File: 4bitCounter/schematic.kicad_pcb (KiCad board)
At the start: 2 copper layers, 20 parts, among them J2 Conn_01x02_Pin, Q1 PN2222A, U1 NE555P, U3 74LS161

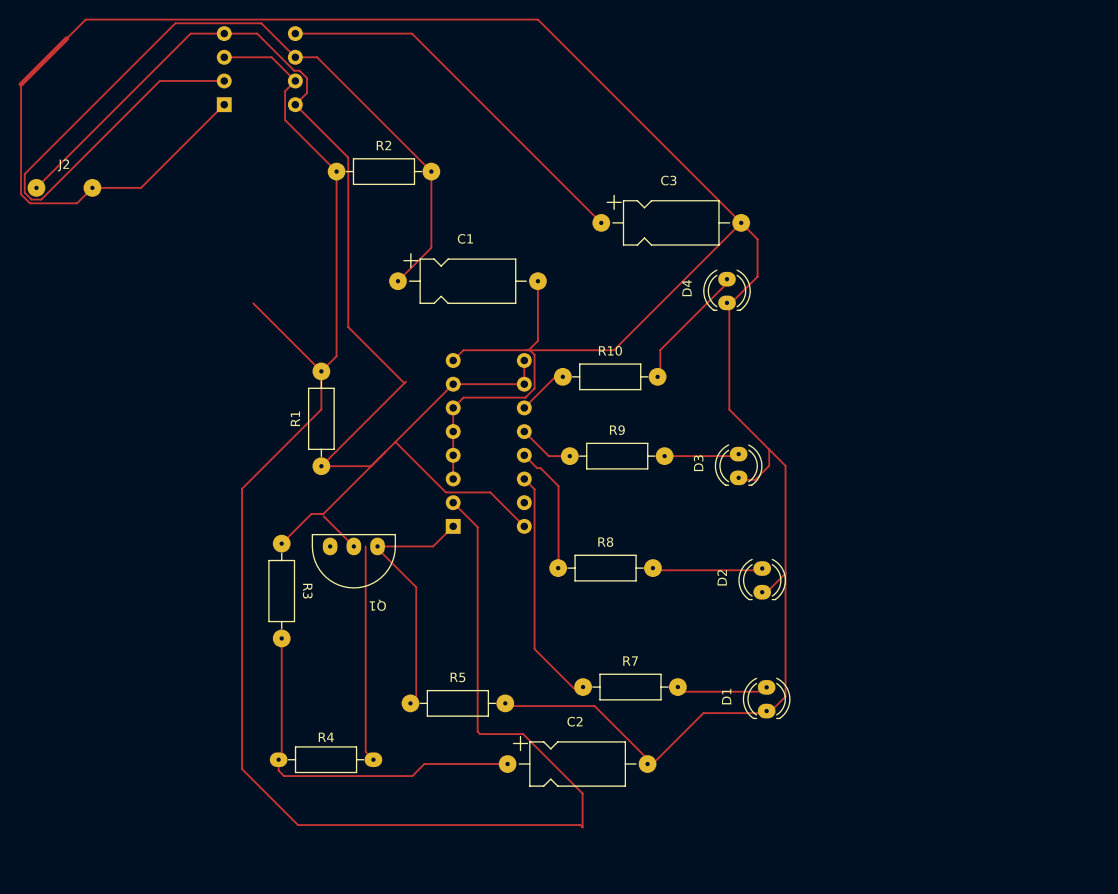
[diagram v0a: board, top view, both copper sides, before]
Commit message: Update footprints and pcb
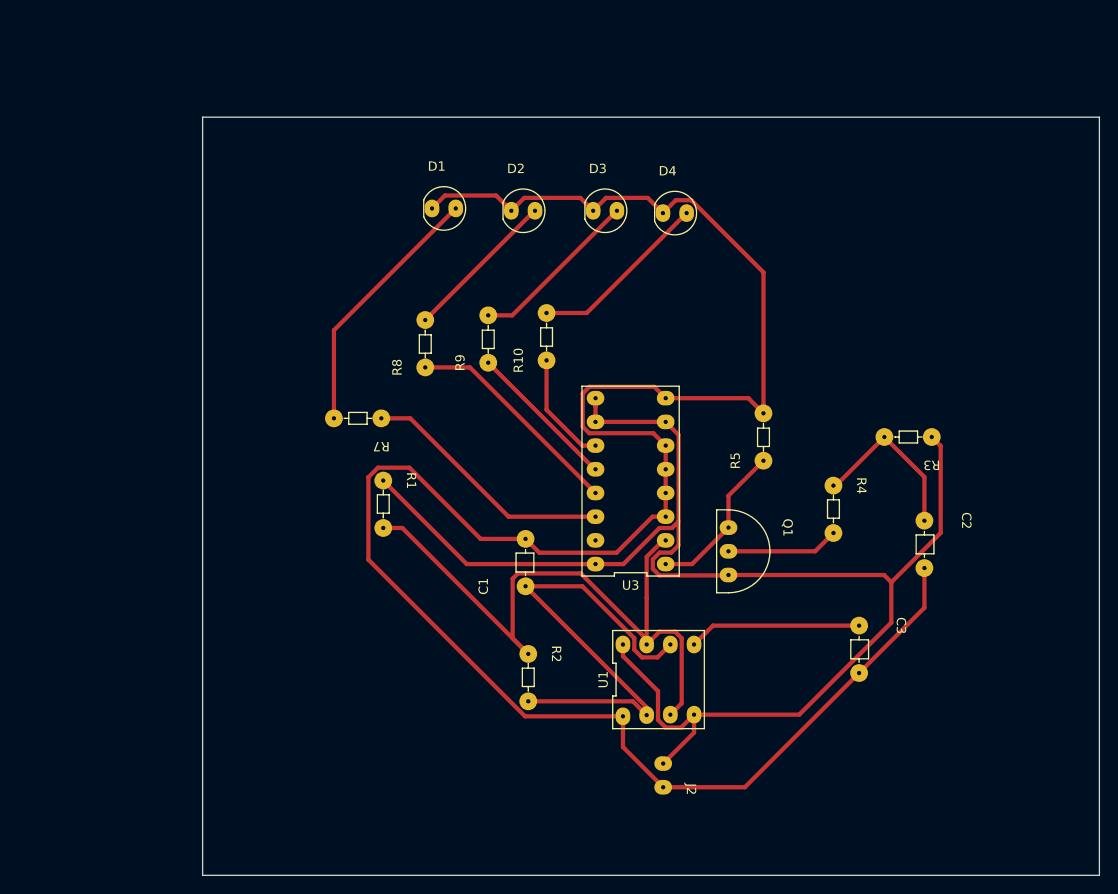
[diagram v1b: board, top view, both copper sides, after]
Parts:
- Q1: footprint CounterProject:transistor -> CounterProject:Transistor
- R4: footprint 4bitCounter:Resistor -> CounterProject:Resistor
- U1: footprint Package_DIP:DIP-8_W7.62mm -> CounterProject:Timer; moved to F.Cu
- U3: footprint Package_DIP:DIP-16_W7.62mm -> CounterProject:CounterChip; moved to F.Cu
- moved J2 89.0 mm to (233.2, 148.9), turned to -90 degrees
- moved U1 78.3 mm to (228.9, 143.9)
- moved R3 71.8 mm to (262.0, 114.0), turned to 180 degrees
- moved R4 66.3 mm to (251.4, 119.2), turned to -90 degrees
- moved D1 64.0 mm to (208.4, 89.5), turned to 0 degrees
- moved R2 53.7 mm to (218.7, 137.2), turned to -90 degrees
- moved D2 48.2 mm to (216.9, 89.7), turned to 0 degrees
- moved C3 47.7 mm to (254.2, 134.2), turned to -90 degrees
- moved C2 45.6 mm to (261.2, 122.9), turned to -90 degrees
- moved R5 42.0 mm to (243.9, 116.5), turned to 90 degrees
- moved R7 39.5 mm to (203.0, 112.0), turned to 180 degrees
- moved Q1 37.7 mm to (240.2, 123.7), turned to -90 degrees
- moved C1 33.3 mm to (218.4, 129.9), turned to 90 degrees
- moved D3 31.8 mm to (225.7, 89.7), turned to 0 degrees
- moved R8 29.1 mm to (207.7, 106.5), turned to 90 degrees
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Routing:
- net Net-(U1-DIS): track 182.0 -> 73.4 mm
- net Net-(D1-K): track 293.0 -> 230.6 mm
- net Net-(U1-THR): track 99.1 -> 52.5 mm
- net Net-(U1-CV): track 41.2 -> 18.5 mm
- net Net-(C2-Pad1): track 40.2 -> 18.4 mm
- net Net-(D1-A): track 10.5 -> 27.9 mm
- net Net-(Q1-B): track 27.8 -> 12.1 mm
- net Net-(J2-Pin_1): track 149.3 -> 161.0 mm
- net Net-(Q1-E): track 27.8 -> 17.1 mm
- net Net-(D3-A): track 7.90 -> 18.4 mm
- net Net-(U3-Q1): track 13.8 -> 23.8 mm
- net Net-(U3-Q2): track 6.26 -> 16.2 mm
- net Net-(D4-A): track 12.8 -> 19.5 mm
- net Net-(U3-Q3): track 6.01 -> 12.1 mm
- net Net-(D2-A): track 12.0 -> 16.6 mm
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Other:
- board outline added: 96.1 x 81.3 mm
